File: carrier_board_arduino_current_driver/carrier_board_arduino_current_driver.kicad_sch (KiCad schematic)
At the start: 13 parts, among them J1 Conn_01x03_Pin, J3 Barrel_Jack, Q1 TIP41, Q2 TIP42, U1 L7805

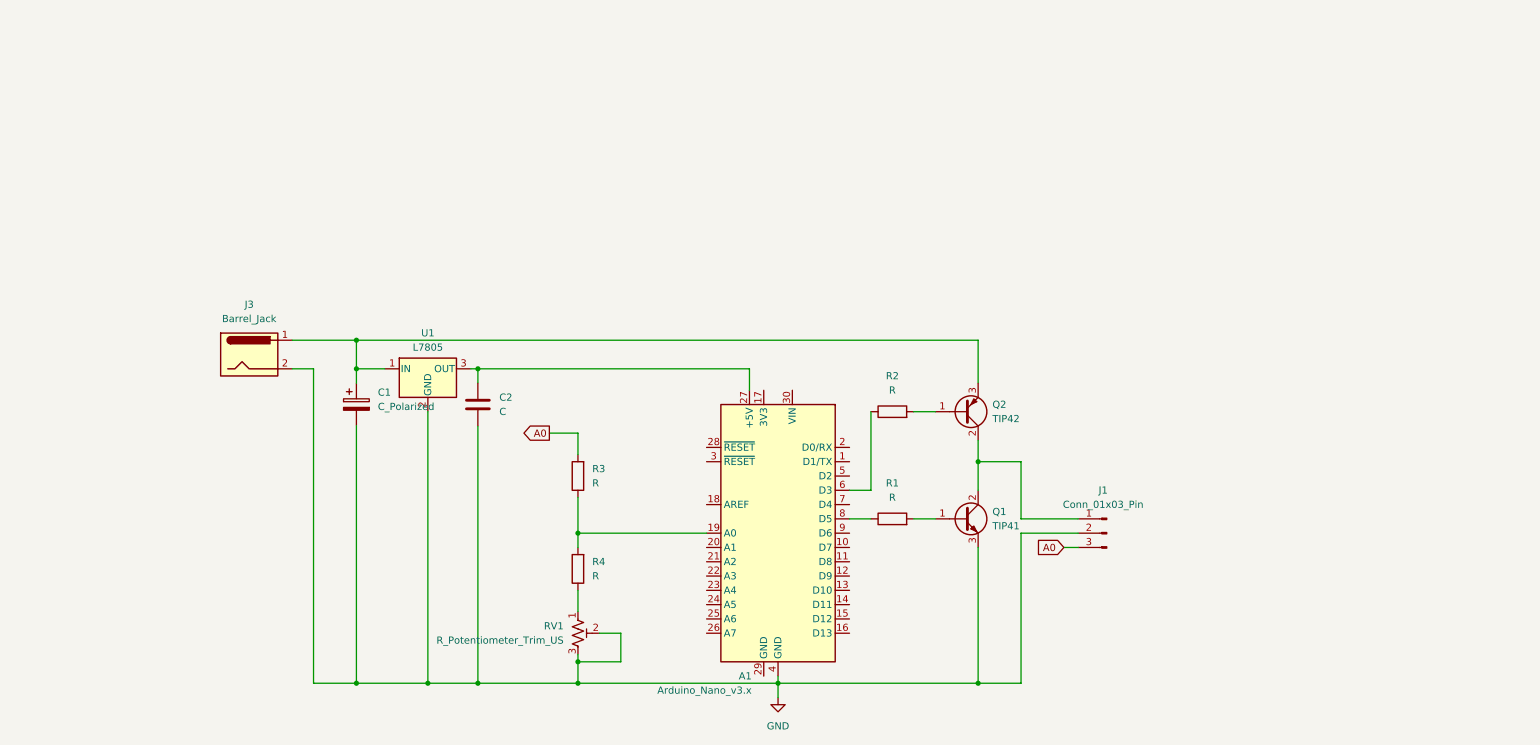
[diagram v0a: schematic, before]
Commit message: v1.0.0
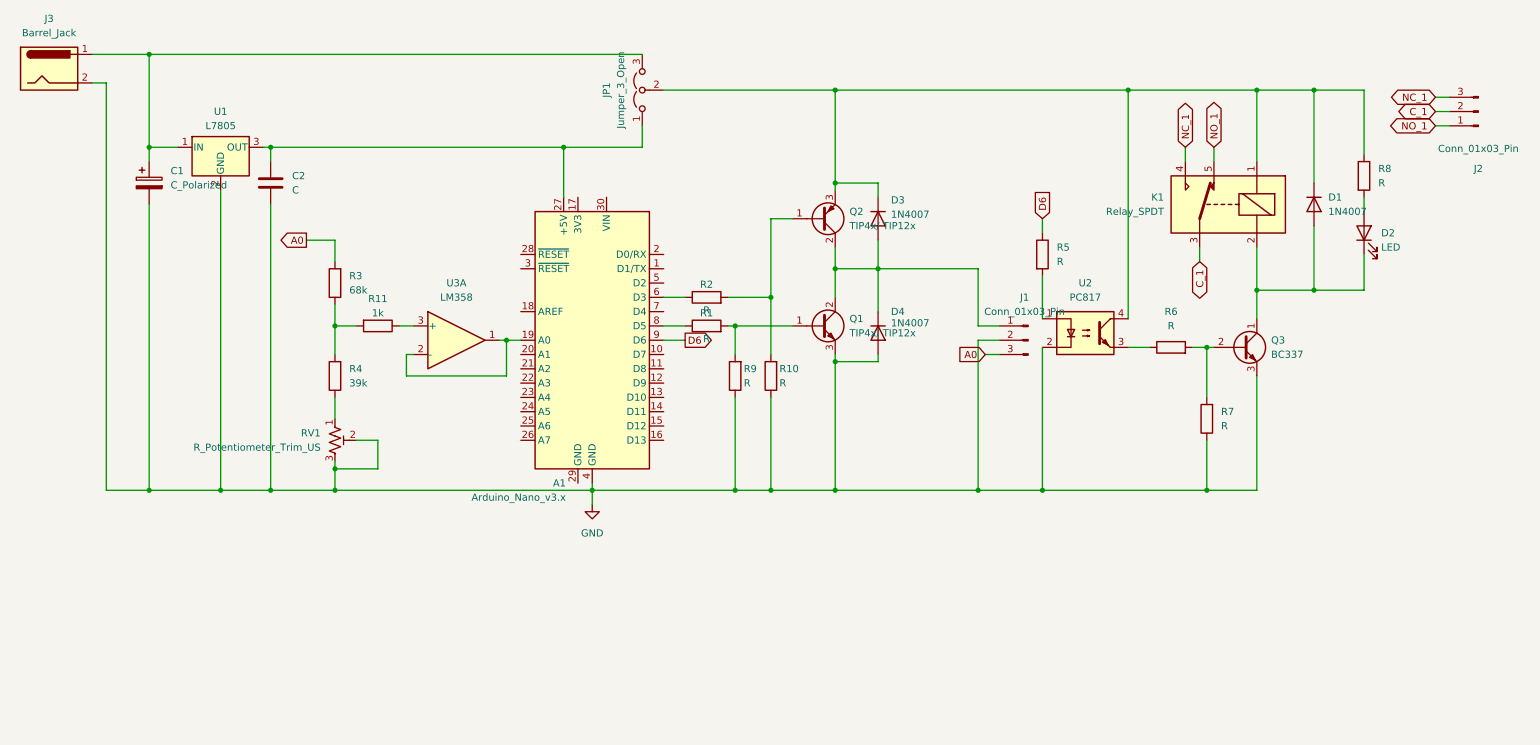
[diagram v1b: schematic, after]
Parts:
- added D1, D3, D4: 1N4007, Diode_THT:D_DO-41_SOD81_P10.16mm_Horizontal, symbol Diode:1N4007
- added D2: LED, LED_THT:LED_D3.0mm, symbol Device:LED
- added J2: Conn_01x03_Pin, TerminalBlock_Phoenix:TerminalBlock_Phoenix_MKDS-1,5-3-5.08_1x03_P5.08mm_Horizontal, symbol Connector:Conn_01x03_Pin
- added JP1: Jumper_3_Open, Connector_PinHeader_2.54mm:PinHeader_1x03_P2.54mm_Vertical, symbol Jumper:Jumper_3_Open
- added K1: Relay_SPDT, Relay_THT:Relay_SPDT_Omron-G5LE-1, symbol Relay:Relay_SPDT
- added Q3: BC337, Package_TO_SOT_THT:TO-92_Inline, symbol Transistor_BJT:BC337
- added R10, R5, R6, R7, R8, R9: R, Resistor_THT:R_Axial_DIN0207_L6.3mm_D2.5mm_P7.62mm_Horizontal, symbol Device:R
- added R11: 1k, Resistor_THT:R_Axial_DIN0207_L6.3mm_D2.5mm_P7.62mm_Horizontal, symbol Device:R
- added U2: PC817, Package_DIP:DIP-4_W7.62mm, symbol Isolator:PC817
- added U3: LM358, Package_DIP:DIP-8_W7.62mm, symbol Amplifier_Operational:LM358
- Q1: value TIP41 -> TIP4x/ TIP12x
- Q2: value TIP42 -> TIP4x/ TIP12x
- R3: value R -> 68k
- R4: value R -> 39k
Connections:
- net GND: now also D4.2 (A), Q3.3 (E), R10.1, R7.1, R9.1, U2.2
- net at J1.1 (Pin_1), Q1.2 (C), Q2.2 (C): now also D3.2 (A), D4.1 (K)
- net at Q1.1 (B), R1.2: now also R9.2
- net at R3.1, R4.2: now also R11.2; no longer A1.19 (A0)
- net at A1.27 (+5V), C2.1, U1.3 (OUT): now also JP1.1 (A)
- net D6: now reaches A1.9 (D6)
- net D6: now also R5.1
- net at C1.1, J3.1, U1.1 (IN): now also JP1.3 (B); no longer Q2.3 (E)
- net at Q2.1 (B), R2.2: now also R10.2
- new net: D1.1 (K), D3.1 (K), JP1.2 (C), K1.1, Q2.3 (E), R8.1, U2.4
- new net: A1.19 (A0), U3.1, U3.2 (-)
- new net: R11.1, U3.3 (+)
- new net: R6.1, U2.3
- new net: Q3.2 (B), R6.2, R7.2
- new net: D1.2 (A), D2.1 (K), K1.2, Q3.1 (C)
- new net: D2.2 (A), R8.2
- new net: R5.2, U2.1
- new net C_1: J2.2 (Pin_2), K1.3
- new net NC_1: J2.3 (Pin_3), K1.4
- new net NO_1: J2.1 (Pin_1), K1.5
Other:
- moved on the sheet: A1, C1, C2, J1, J3, Q1, Q2, R1, R2, R3, R4, RV1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
